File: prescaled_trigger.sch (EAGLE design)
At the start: 41 parts, among them T1 2N2369, U1 MC100EP196FAG, U2 MC100EPT22DG, X1 BU-SMA-H, X2 BU-SMA-H, X3 BU-SMA-H, X4 BU-SMA-H

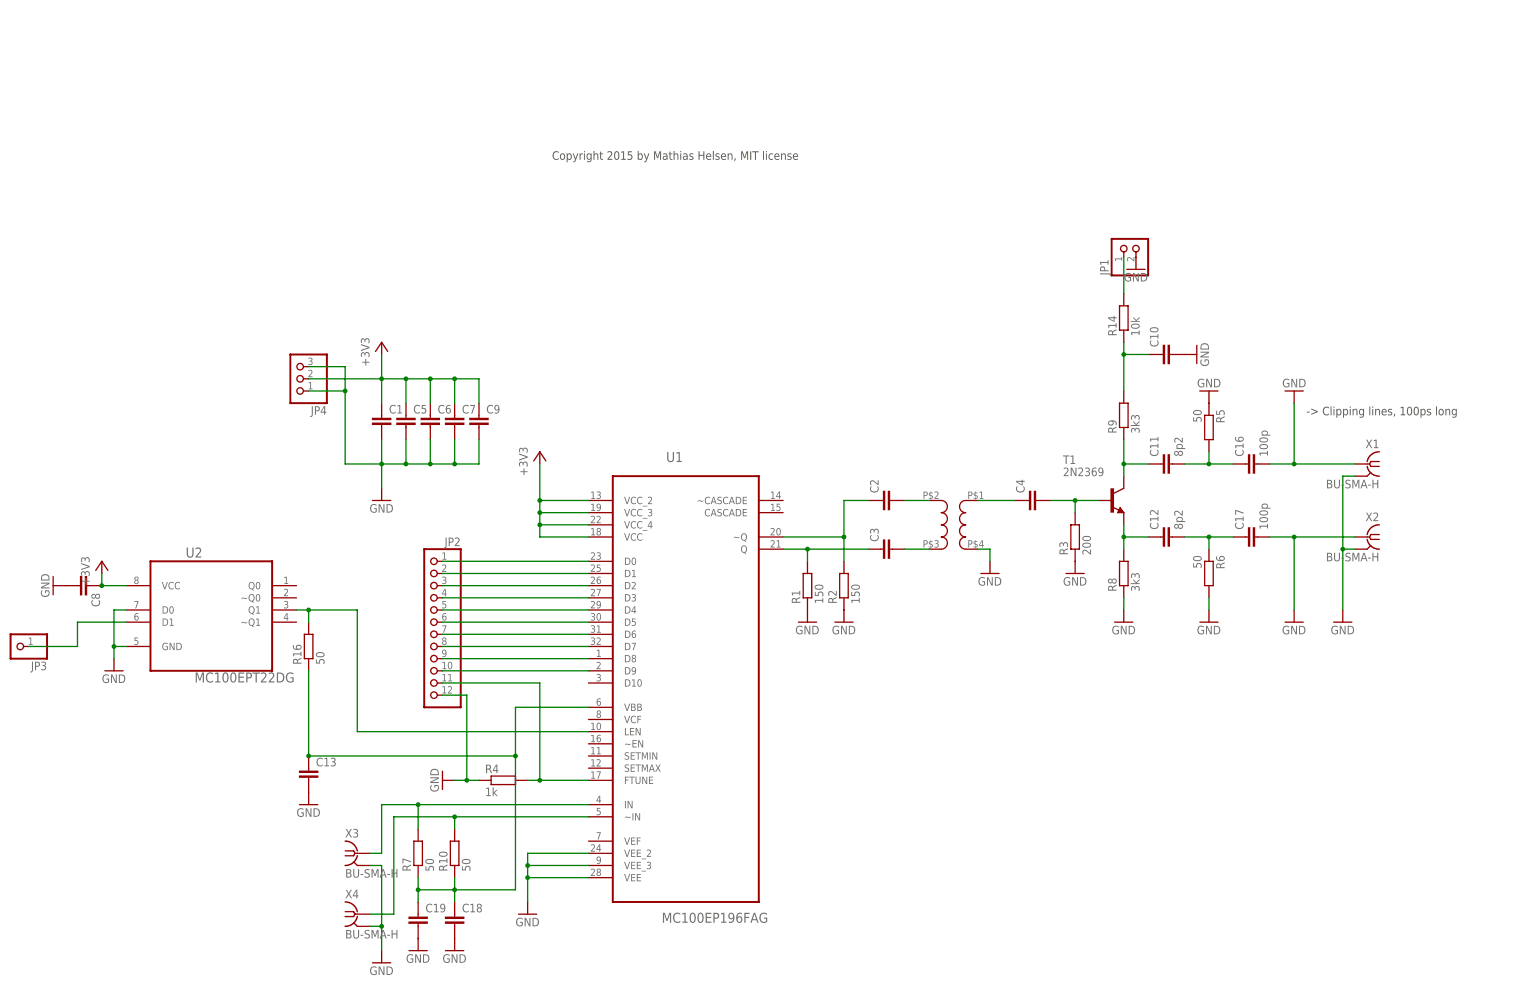
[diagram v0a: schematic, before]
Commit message: added prescaled trigger, Work In Progress
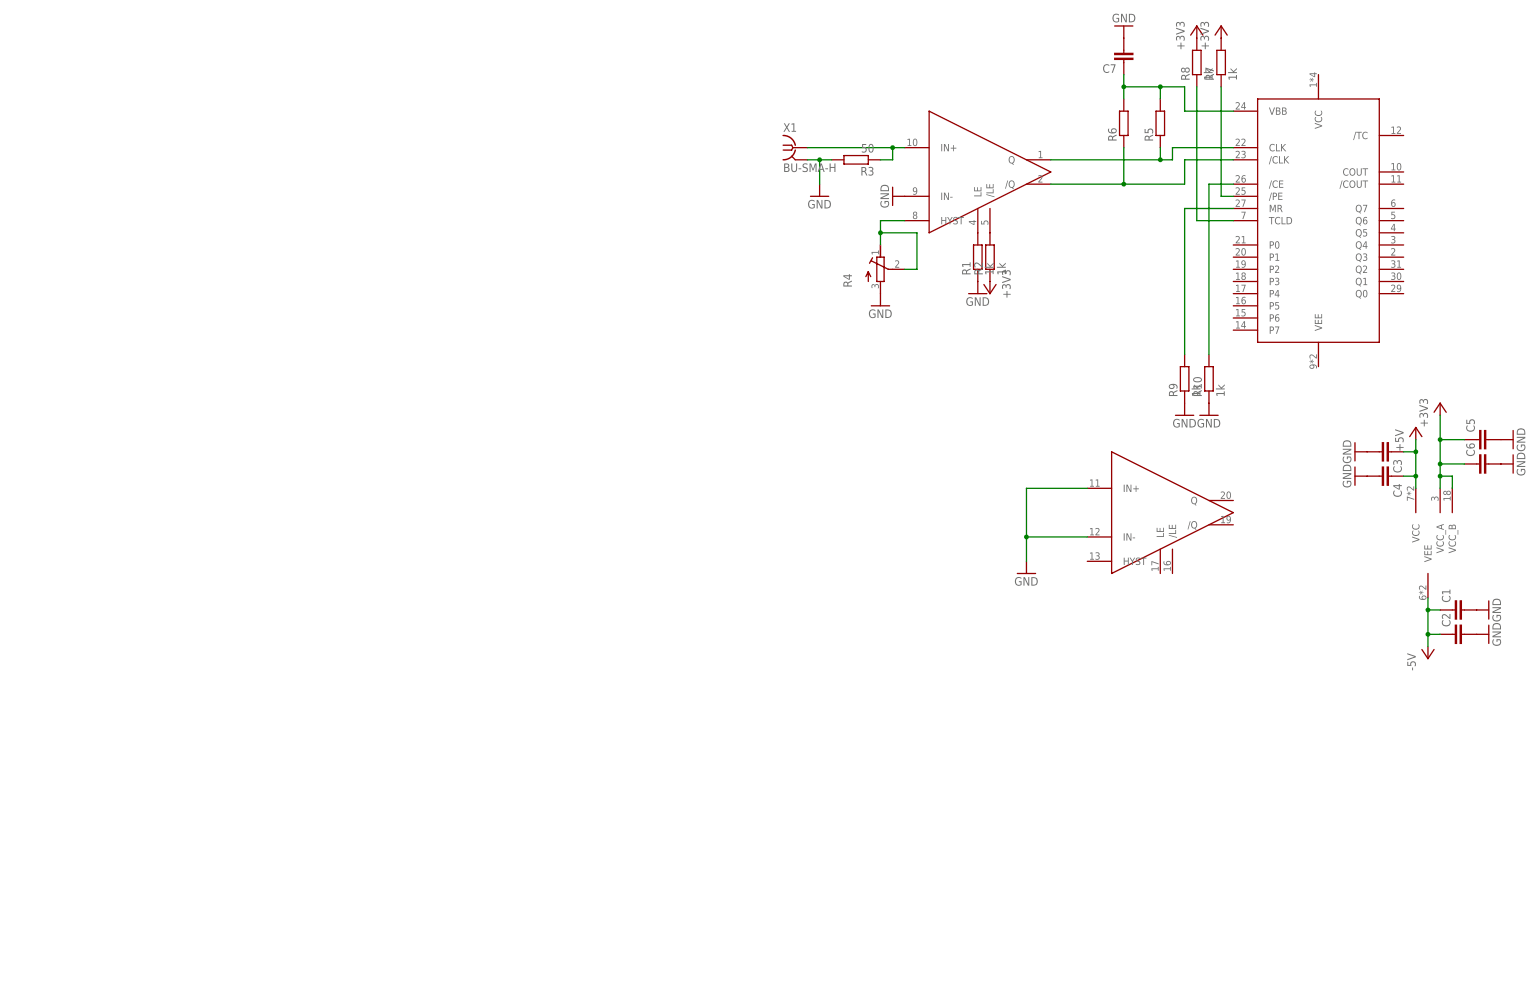
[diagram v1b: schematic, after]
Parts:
- removed C10, C13, C18, C19, C8: (no value), resistor:C-EUC0805
- removed C11, C12: 8p2, resistor:C-EUC0603
- removed C16, C17: 100p, resistor:C-EUC0603
- removed C9: (no value), resistor:C-EUC1206
- removed JP1: (no value), pinhead:PINHD-1X2
- removed JP2: (no value), pinhead:PINHD-1X12
- removed JP3: (no value), pinhead:PINHD-1X1
- removed JP4: (no value), pinhead:PINHD-1X3
- removed R14: 10k, resistor:R-EU_R0805
- removed R16: 50, resistor:R-EU_R0805
- removed T1: 2N2369, transistor-neu-to92:2N2369
- removed U1: MC100EP196FAG, MC100EP196:MC100EP196FAG
- removed U2: MC100EPT22DG, MC100EPT22:MC100EPT22DG
- removed X2, X3, X4: BU-SMA-H, con-coax:BU-SMA-H
- added U$2: MC100EP016, MC100EP016:MC100EP016
- R1, R2: value 150 -> 1k; device resistor:R-EU_R0805 -> resistor:R-EU_M0805
- R10, R7: value 50 -> 1k; device resistor:R-EU_R0805 -> resistor:R-EU_M0805
- R3: value 200 -> 50; device resistor:R-EU_R0805 -> resistor:R-EU_M0805
- R4: value 1k -> (none); device resistor:R-EU_R0805 -> resistor:R-TRIMMT18
- R5, R6: value 50 -> (none); device resistor:R-EU_R0603 -> resistor:R-EU_M0805
- R8, R9: value 3k3 -> 1k; device resistor:R-EU_R0805 -> resistor:R-EU_M0805
- U$1: value JA4220 -> MAX9601; device \cct:JA4220 -> MAX9601:MAX9601
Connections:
- removed net N$14: JP2.4, U1.D3
- removed net N$15: JP2.5, U1.D4
- removed net N$16: JP2.6, U1.D5
- removed net N$17: JP2.7, U1.D6
- removed net N$18: JP2.8, U1.D7
- removed net N$19: C10.1, R14.1, R9.2
- removed net N$20: JP2.9, U1.D8
- removed net N$21: JP2.10, U1.D9
- removed net N$22: JP1.1, R14.2
- removed net N$26: C11.2, C16.1, R5.2
- removed net N$27: C12.2, C17.1, R6.1
- removed net N$30: R10.2, U1.~IN, X4.1
- removed net N$31: R7.2, U1.IN, X3.1
- removed net N$32: R16.2, U1.LEN, U2.Q1
- removed net N$34: JP3.1, U2.D1
- removed net N$8: JP2.2, U1.D1
- removed net N$9: JP2.11, R4.2, U1.FTUNE
- removed net VBB: C13.1, C18.1, C19.1, R10.1, R16.1, R7.1, U1.VBB
- new net +5V: C3.1, C4.1, U$1G$3.VCC
- new net -5V: C1.1, C2.1, U$1G$3.VEE
- new net N$13: R10.2, U$2./CE
- net +3V3: now also R2.1, R7.2, R8.2, U$1G$3.VCC_A, U$1G$3.VCC_B; no longer C1.1, C7.1, C8.1, C9.1, JP4.2, U1.VCC, U1.VCC_2, U1.VCC_3, U1.VCC_4, U2.VCC
- net GND: now also C2.2, C3.2, C4.2, R10.1, R3.2, R4.E, R9.1, U$1G$1.IN-, U$1G$2.IN+, U$1G$2.IN-; no longer C10.2, C13.2, C16.2, C17.2, C18.2, C19.2, C8.2, C9.2, JP1.2, JP2.12, JP4.1, JP4.3, R2.1, R3.1, R4.1, R5.1, R6.2, R8.1, U$1.P$4, U1.VEE, U1.VEE_2, U1.VEE_3, U2.D0, U2.GND, X1.1, X2.1, X2.2, X3.2, X4.2
- net N$1: now also R1.2, U$1G$1.LE; no longer JP2.1, U1.D0
- net N$10: now also R8.1, U$2.TCLD; no longer JP2.3, U1.D2
- net N$11: now also R7.1, U$2./PE; no longer C11.1, R9.1, T1.C
- net N$12: now also R9.2, U$2.MR; no longer C12.1, R8.2, T1.E
- net N$2: now also R2.2, U$1G$1./LE; no longer C3.1, R1.2, U1.Q
- net N$3: now also R3.1, U$1G$1.IN+, X1.1; no longer C2.1, R2.2, U1.~Q
- net N$4: now also R4.A, R4.S, U$1G$1.HYST; no longer C2.2, U$1.P$2
- net N$5: now also R5.1, U$1G$1.Q, U$2.CLK; no longer C3.2, U$1.P$3
- net N$6: now also R6.1, U$1G$1./Q, U$2./CLK; no longer C4.1, U$1.P$1
- net N$7: now also C7.1, R5.2, R6.2, U$2.VBB; no longer C4.2, R3.2, T1.B
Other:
- note removed: "-> Clipping lines, 100ps long"
- note removed: "Copyright 2015 by Mathias Helsen, MIT license"
- moved on the sheet: C1, C2, C3, C4, C5, C6, C7, R1, R10, R2, R3, R5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
